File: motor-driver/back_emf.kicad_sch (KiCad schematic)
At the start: 7 parts, among them U15 LM397

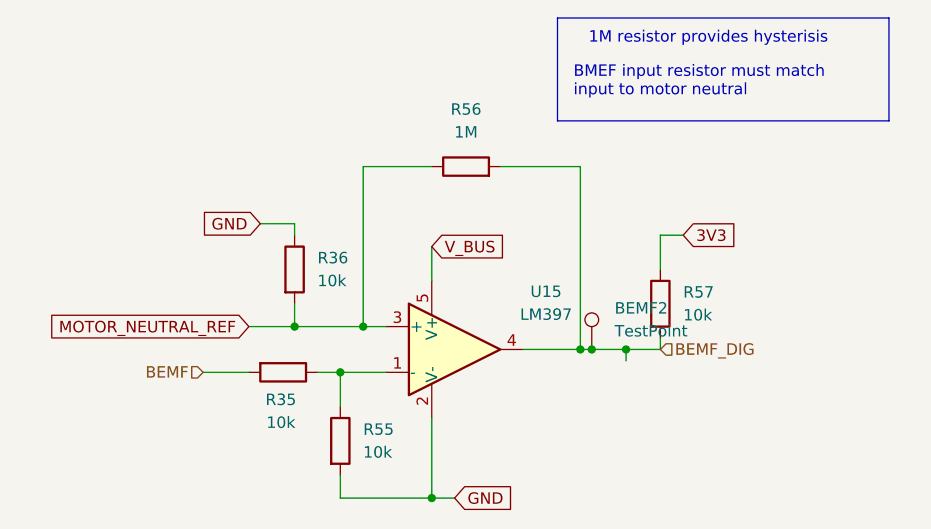
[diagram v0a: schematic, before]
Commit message: added test points
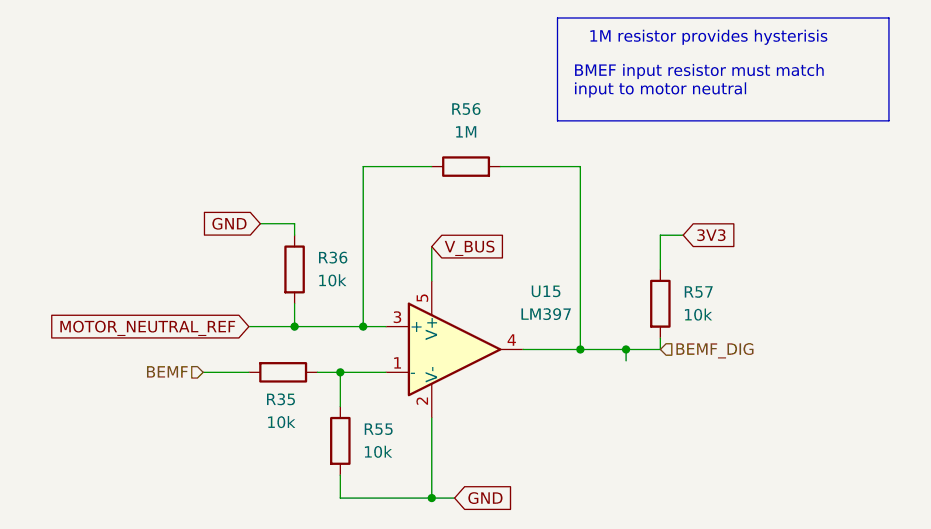
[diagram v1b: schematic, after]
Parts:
- removed BEMF2: TestPoint, TestPoint:TestPoint_Loop_D1.80mm_Drill1.0mm_Beaded, symbol Connector:TestPoint
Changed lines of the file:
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@@
-	)
-	(junction
-		(at 160.02 100.33)
-		(diameter 0)
-		(color 0 0 0 0)
 	)
 	(junction
@@
 	(wire
 		(pts
-			(xy 160.02 100.33) (xy 163.83 100.33)
-		)
-		(stroke
-			(width 0)
-			(type default)
-		)
-	)
-	(wire
-		(pts
 			(xy 142.24 88.9) (xy 142.24 92.71)
 		)
@@
 	(wire
 		(pts
-			(xy 158.75 100.33) (xy 160.02 100.33)
+			(xy 158.75 100.33) (xy 163.83 100.33)
 		)
 		(stroke
@@
 					(unit 1)
 				)
-			)
-		)
-	)
-	(symbol
-		(lib_id "Connector:TestPoint")
-		(at 160.02 100.33 0)
-		(unit 1)
-		(exclude_from_sim no)
-		(in_bom no)
-		(on_board yes)
-		(dnp no)
-		(fields_autoplaced yes)
-		(property "Reference" "BEMF2"
-			(at 162.56 95.7579 0)
-			(effects
-				(font
-					(size 1.27 1.27)
-				)
-				(justify left)
-			)
-		)
-		(property "Value" "TestPoint"
-			(at 162.56 98.2979 0)
-			(effects
-				(font
-					(size 1.27 1.27)
-				)
-				(justify left)
-			)
-		)
-		(property "Footprint" "TestPoint:TestPoint_Loop_D1.80mm_Drill1.0mm_Beaded"
-			(at 165.1 100.33 0)
-			(effects
-				(font
-					(size 1.27 1.27)
-				)
-				(hide yes)
-			)
-		)
-		(property "Datasheet" "~"
-			(at 165.1 100.33 0)
-			(effects
-				(font
-					(size 1.27 1.27)
-				)
-				(hide yes)
-			)
-		)
-		(property "Description" "test point"
-			(at 160.02 100.33 0)
-			(effects
-				(font
-					(size 1.27 1.27)
-				)
-				(hide yes)
-			)
-		)
-		(pin "1"
-		)
-		(instances
-			(project "motor-driver"
-				(path "/2980fc7e-b297-4843-ba9f-cceafa384b2f/d36b7053-ee22-4492-bdec-8a6a56460e2b/5dcb47c1-5cbd-4c06-ae20-6bf4ebc0293f"
-					(reference "BMEF1")
-					(unit 1)
-				)
-				(path "/2980fc7e-b297-4843-ba9f-cceafa384b2f/d36b7053-ee22-4492-bdec-8a6a56460e2b/d55dfac5-5848-47fb-8309-2ae121a74f55"
-					(reference "BEMF3")
-					(unit 1)
-				)
-				(path "/2980fc7e-b297-4843-ba9f-cceafa384b2f/d36b7053-ee22-4492-bdec-8a6a56460e2b/e5439fff-5f30-49ba-87ec-c8b9c8d18afa"
-					(reference "BEMF2")
-					(unit 1)
-				)
